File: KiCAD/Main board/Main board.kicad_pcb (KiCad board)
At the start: 2 copper layers, 190 x 125 mm, 356 parts, among them J1 Conn_01x03, J10 Conn_01x03, J11 Conn_01x03, J12 Conn_01x03, J13 Conn_01x02, J14 Conn_01x02, J15 Conn_01x06, J16 Conn_01x02, J17 Conn_01x02, J18 Conn_01x05, J19 Conn_01x05, J2 Conn_01x03, J20 Conn_01x05, J21 Conn_01x05, J3 Conn_01x02, J4 Conn_01x02, J5 Conn_01x03, J6 Conn_01x02, J7 Conn_01x03, J8 Conn_01x02, J9 Conn_01x03, K1 EA2-12NU, K2 EA2-12NU, Q1 BC847, Q2 BC847, U1 PCM1789, U10 PCM1789, U11 OPA1632DR, U12 LIN_REG_±5V, U13 LIN_REG_±5V, U14 LIN_REG_±12V, U15 LIN_REG_±12V, U16 PCM1789, U17 OPA1632DR, U18 12V, U19 5V, U2 LM4562, U20 8V, U21 15V, U22 OPA1632DR, U23 OPA1632DR, U24 LM4562, U25 OPA1632DR, U26 LM4562, U27 OPA1632DR, U28 12V, U29 AP2111H-3.3TRG1, U3 OPA1632DR, U30 LM4562, U31 AP2111H-3.3TRG1, U32 LM4562, U33 OPA1632DR, U34 TL072, U35 TL072, U4 OPA1632DR, U5 OPA1632DR, U6 LM4562, U7 PCM1804, U9 SEPIC_-15V_LT3579

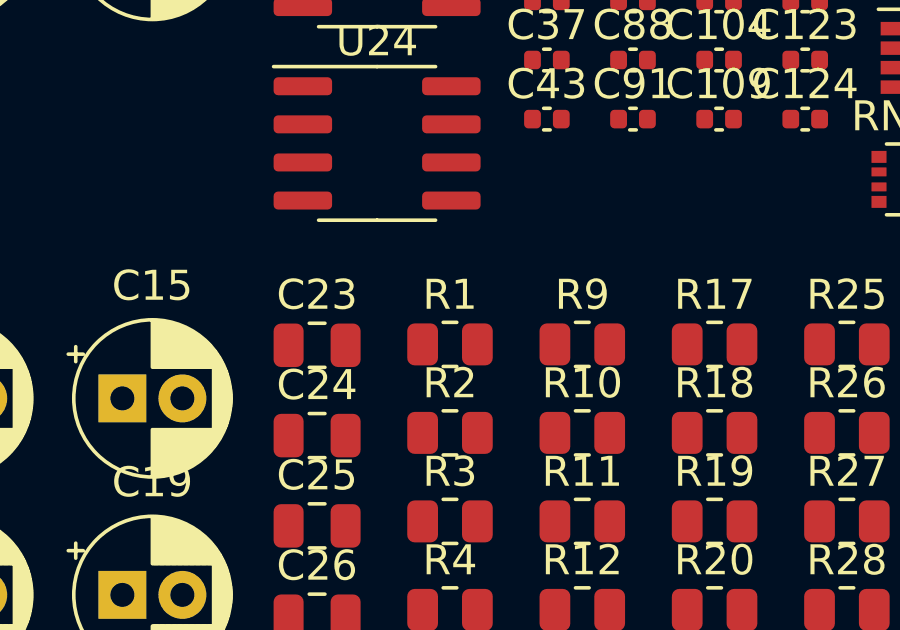
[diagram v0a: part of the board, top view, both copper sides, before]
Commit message: Worked on main board
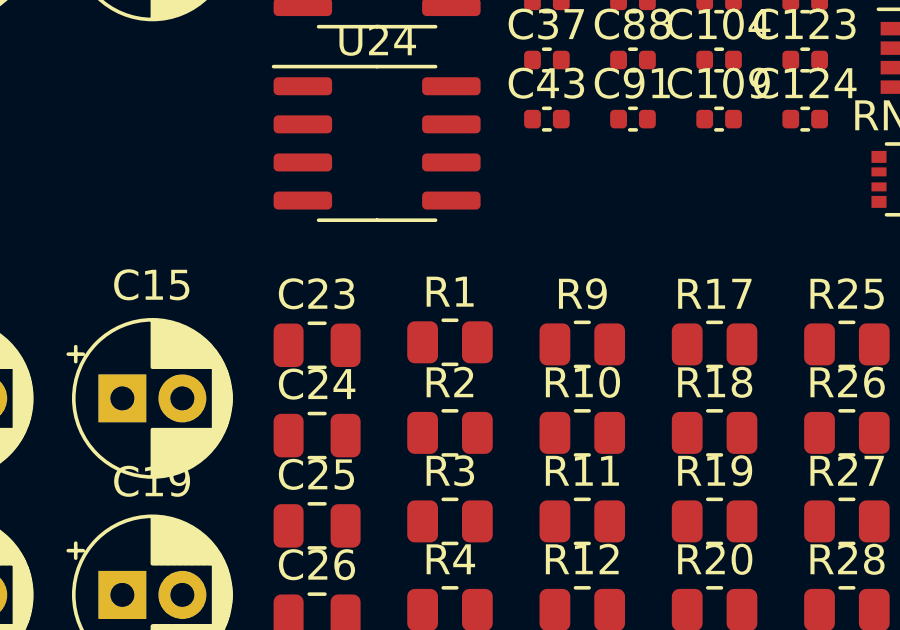
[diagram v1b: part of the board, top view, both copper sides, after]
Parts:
- moved R1 0.07 mm to (330.4, 67.0)
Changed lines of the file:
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@@
   )
   (footprint "Resistor_SMD:R_0805_2012Metric" (layer "F.Cu")
-    (at 330.45 67.07)
+    (at 330.45 67)
     (descr "Resistor SMD 0805 (2012 Metric), square (rectangular) end terminal, IPC_7351 nominal, (Body size source: IPC-SM-782 page 72, https://www.pcb-3d.com/wordpress/wp-content/uploads/ipc-sm-782a_amendment_1_and_2.pdf), generated with kicad-footprint-generator")
     (tags "resistor")
